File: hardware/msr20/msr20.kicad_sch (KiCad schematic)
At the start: 13 parts, among them U1 RF-BPF, U2 BGA616, U3 ADE-1+, U4 AD7478, U5 Pico

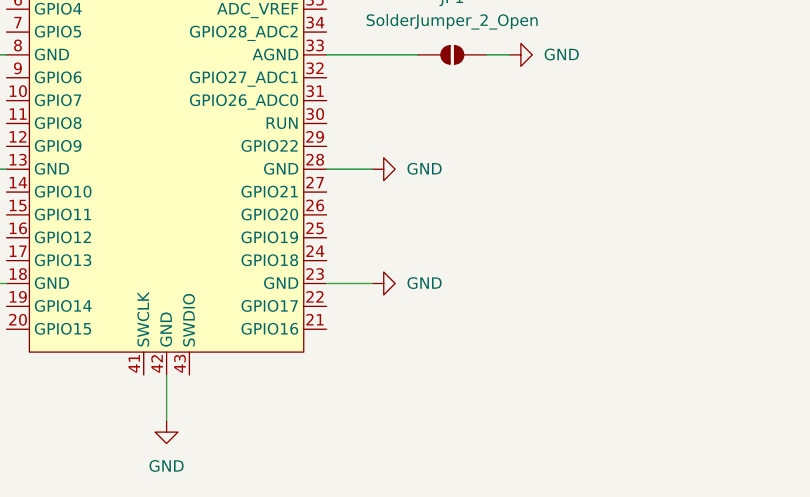
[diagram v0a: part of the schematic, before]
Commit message: save
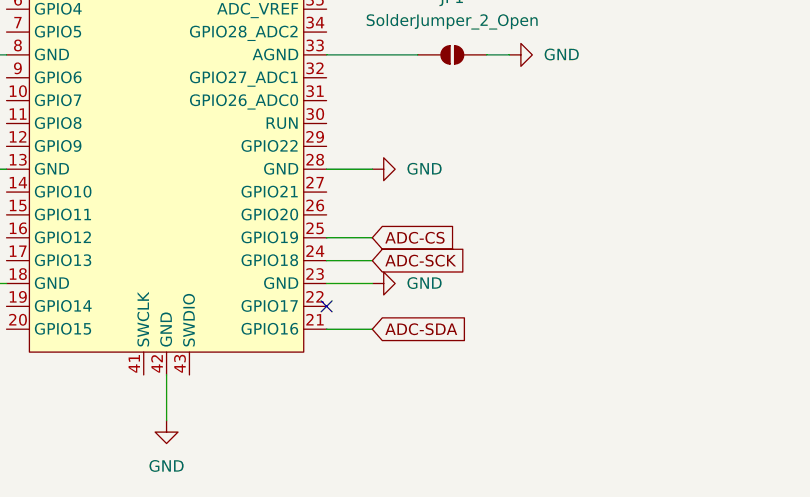
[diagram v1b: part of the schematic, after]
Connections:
- net ADC-CS: now also U5.25 (GPIO19)
- net ADC-SCK: now also U5.24 (GPIO18)
- net ADC-SDA: now also U5.21 (GPIO16)
- no-connect marks 0 -> 1
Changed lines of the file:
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@@
 		(color 0 0 0 0)
 	)
+	(no_connect
+		(at 93.98 173.99)
+	)
 	(wire
 		(pts
@@
 	(wire
 		(pts
+			(xy 93.98 176.53) (xy 99.06 176.53)
+		)
+		(stroke
+			(width 0)
+			(type default)
+		)
+	)
+	(wire
+		(pts
 			(xy 60.96 72.39) (xy 60.96 74.93)
 		)
@@
 	(wire
 		(pts
+			(xy 93.98 166.37) (xy 99.06 166.37)
+		)
+		(stroke
+			(width 0)
+			(type default)
+		)
+	)
+	(wire
+		(pts
 			(xy 204.47 71.12) (xy 207.01 71.12)
 		)
@@
 		(pts
 			(xy 195.58 55.88) (xy 195.58 58.42)
+		)
+		(stroke
+			(width 0)
+			(type default)
+		)
+	)
+	(wire
+		(pts
+			(xy 93.98 168.91) (xy 99.06 168.91)
 		)
 		(stroke
@@
 		)
 	)
+	(global_label "ADC-SDA"
+		(shape input)
+		(at 99.06 176.53 0)
+		(fields_autoplaced yes)
+		(effects
+			(font
+				(size 1.27 1.27)
+			)
+			(justify left)
+		)
+		(property "Intersheetrefs" "${INTERSHEET_REFS}"
+			(at 110.8143 176.53 0)
+			(effects
+				(font
+					(size 1.27 1.27)
+				)
+				(justify left)
+				(hide yes)
+			)
+		)
+	)
 	(global_label "RF-IN"
 		(shape input)
@@
 	)
 	(global_label "ADC-CS"
+		(shape input)
+		(at 99.06 166.37 0)
+		(fields_autoplaced yes)
+		(effects
+			(font
+				(size 1.27 1.27)
+			)
+			(justify left)
+		)
+		(property "Intersheetrefs" "${INTERSHEET_REFS}"
+			(at 109.7257 166.37 0)
+			(effects
+				(font
+					(size 1.27 1.27)
+				)
+				(justify left)
+				(hide yes)
+			)
+		)
+	)
+	(global_label "ADC-CS"
 		(shape output)
 		(at 207.01 71.12 0)
@@
 			(effects
 				(font
+					(size 1.27 1.27)
+				)
+				(justify left)
+				(hide yes)
+			)
+		)
+	)
+	(global_label "ADC-SCK"
+		(shape input)
+		(at 99.06 168.91 0)
+		(fields_autoplaced yes)
+		(effects
+			(font
+				(size 1.27 1.27)
+			)
+			(justify left)
+		)
+		(property "Intersheetrefs" "${INTERSHEET_REFS}"
+			(at 110.9957 168.91 0)
+			(effects
+				(font
